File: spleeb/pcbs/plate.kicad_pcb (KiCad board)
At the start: 2 copper layers, 165.7 x 121.7 mm, 10 parts

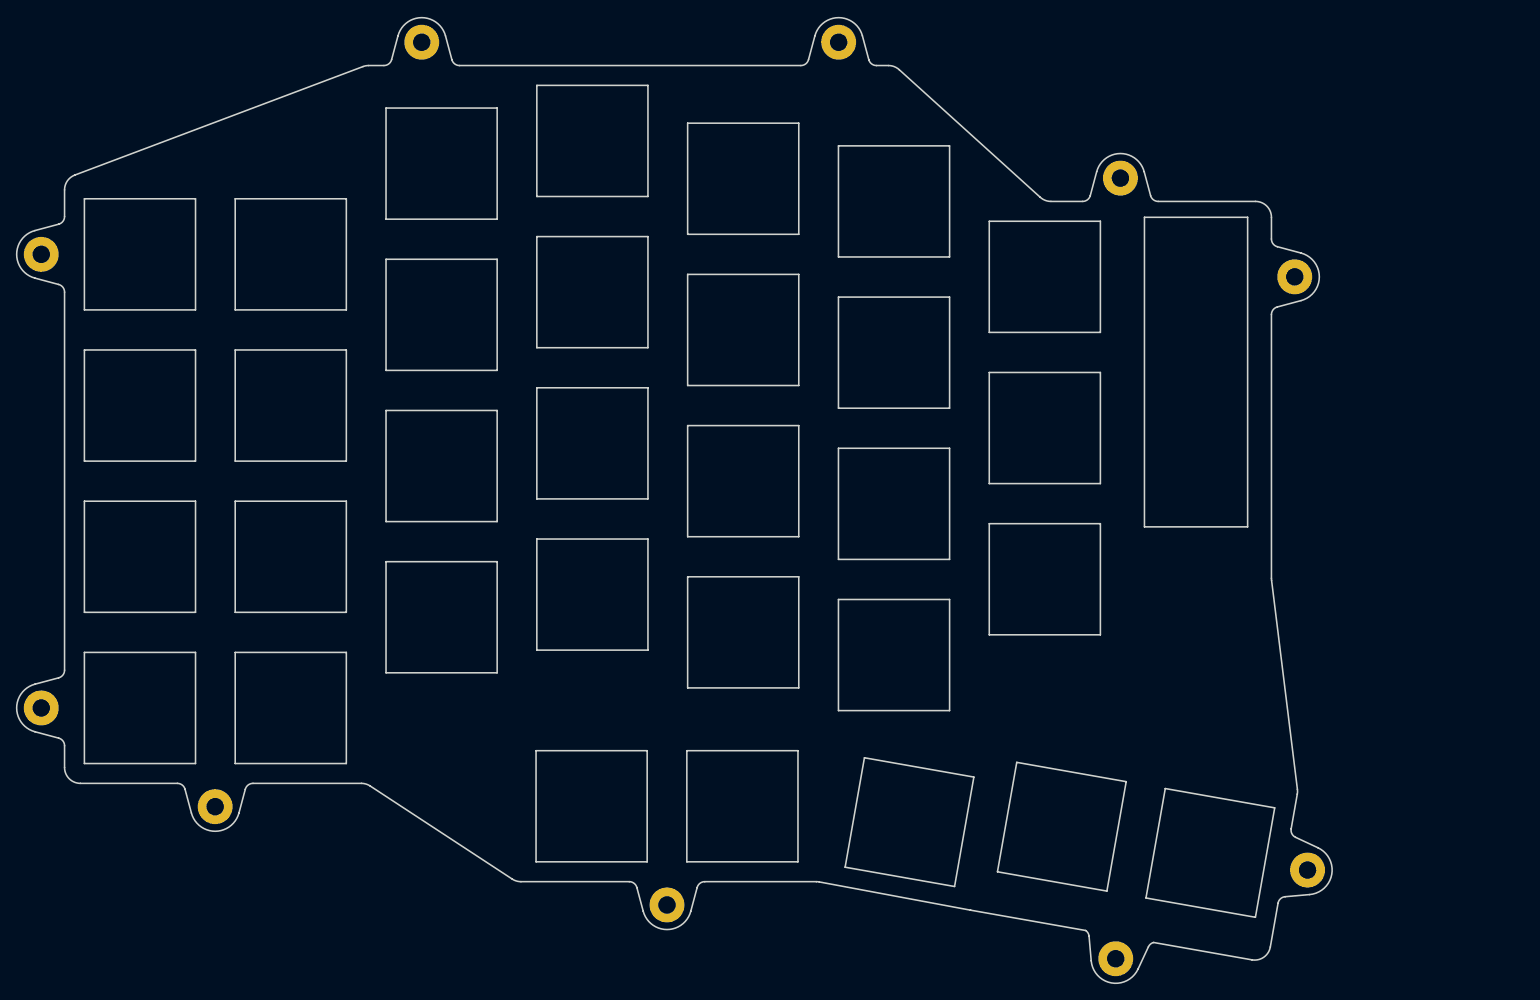
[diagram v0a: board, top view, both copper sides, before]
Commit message: address issues after 3d model test and build with new build changes
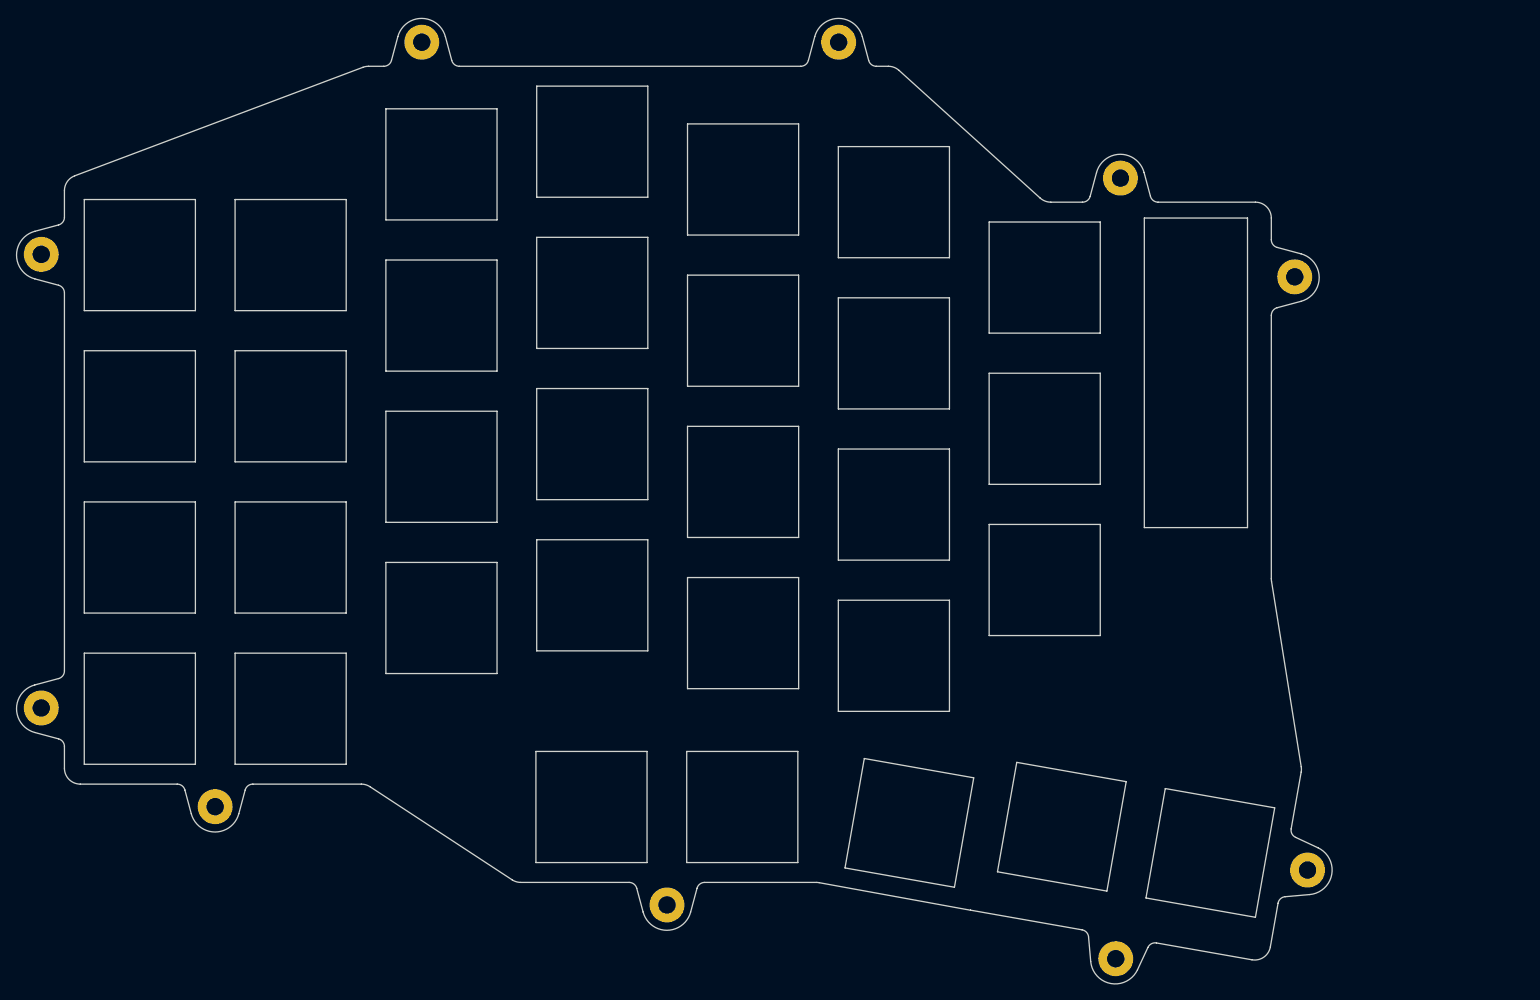
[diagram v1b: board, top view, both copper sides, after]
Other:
- board size 165.7 x 121.7 mm -> 165.7 x 121.6 mm

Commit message: regenerate files
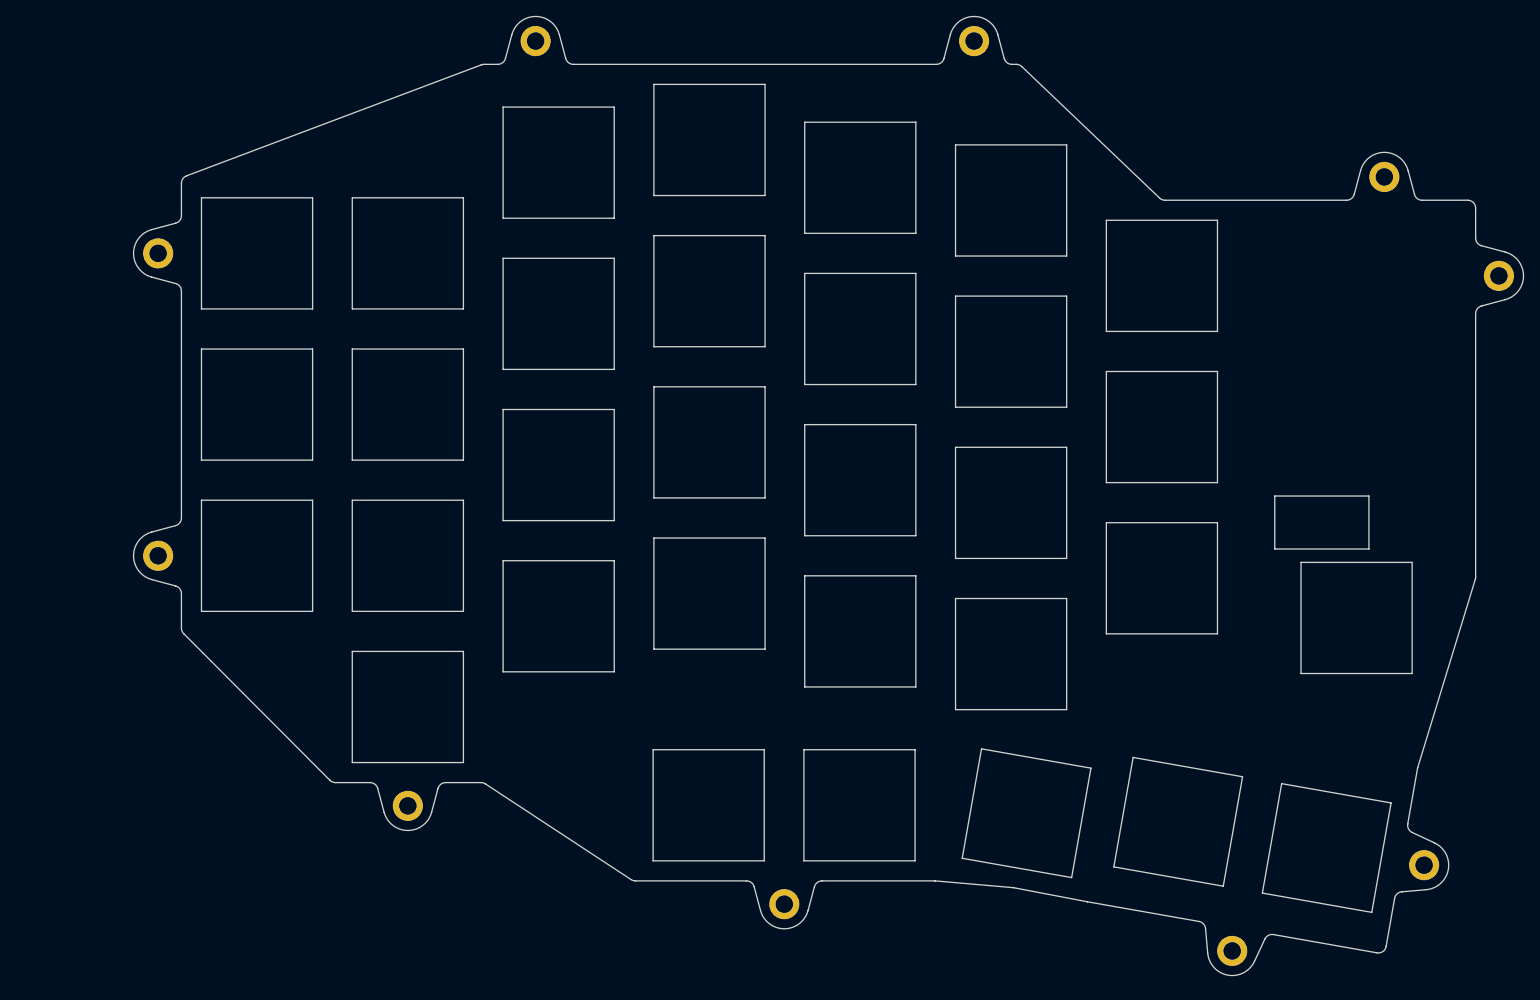
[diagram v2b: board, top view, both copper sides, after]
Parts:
- removed ?: , 
- removed the REF** at (48.3, 119.3)
- removed the REF** at (48.3, 62.2)
- removed the REF** at (148.8, 35.5)
- removed the REF** at (127.1, 144.2)
- removed the REF** at (183.7, 150.9)
- removed the REF** at (70.2, 131.8)
- removed the REF** at (96.2, 35.5)
- removed the REF** at (207.8, 139.8)
- removed the REF** at (206.2, 65.0)
- added REF**: MountingHole_2.2mm_M2_DIN965_Pad, MountingHole:MountingHole_2.2mm_M2_DIN965_Pad, F.Cu at (141.9, 144.1)
- added REF**: MountingHole_2.2mm_M2_DIN965_Pad, MountingHole:MountingHole_2.2mm_M2_DIN965_Pad, F.Cu at (63.0, 100.2)
- added REF**: MountingHole_2.2mm_M2_DIN965_Pad, MountingHole:MountingHole_2.2mm_M2_DIN965_Pad, F.Cu at (217.5, 52.4)
- added REF**: MountingHole_2.2mm_M2_DIN965_Pad, MountingHole:MountingHole_2.2mm_M2_DIN965_Pad, F.Cu at (165.8, 35.3)
- added REF**: MountingHole_2.2mm_M2_DIN965_Pad, MountingHole:MountingHole_2.2mm_M2_DIN965_Pad, F.Cu at (94.5, 131.7)
- added REF**: MountingHole_2.2mm_M2_DIN965_Pad, MountingHole:MountingHole_2.2mm_M2_DIN965_Pad, F.Cu at (198.4, 150.0)
- added REF**: MountingHole_2.2mm_M2_DIN965_Pad, MountingHole:MountingHole_2.2mm_M2_DIN965_Pad, F.Cu at (110.6, 35.3)
- added REF**: MountingHole_2.2mm_M2_DIN965_Pad, MountingHole:MountingHole_2.2mm_M2_DIN965_Pad, F.Cu at (63.0, 62.1)
- added REF**: MountingHole_2.2mm_M2_DIN965_Pad, MountingHole:MountingHole_2.2mm_M2_DIN965_Pad, F.Cu at (232.0, 64.9)
- added REF**: MountingHole_2.2mm_M2_DIN965_Pad, MountingHole:MountingHole_2.2mm_M2_DIN965_Pad, F.Cu at (222.5, 139.1)
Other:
- board size 165.7 x 121.6 mm -> 175.1 x 120.8 mm
